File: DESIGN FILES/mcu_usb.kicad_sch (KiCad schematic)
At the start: 26 parts, among them J401 YTC-TC16S-28, Q401 MMBT3904, Q402 MMBT3904, SW401 TS-1187A-B-A-B, U401 ESP32-WROVER-E-N4R8, U402 CP2102N-A02-GQFN28R

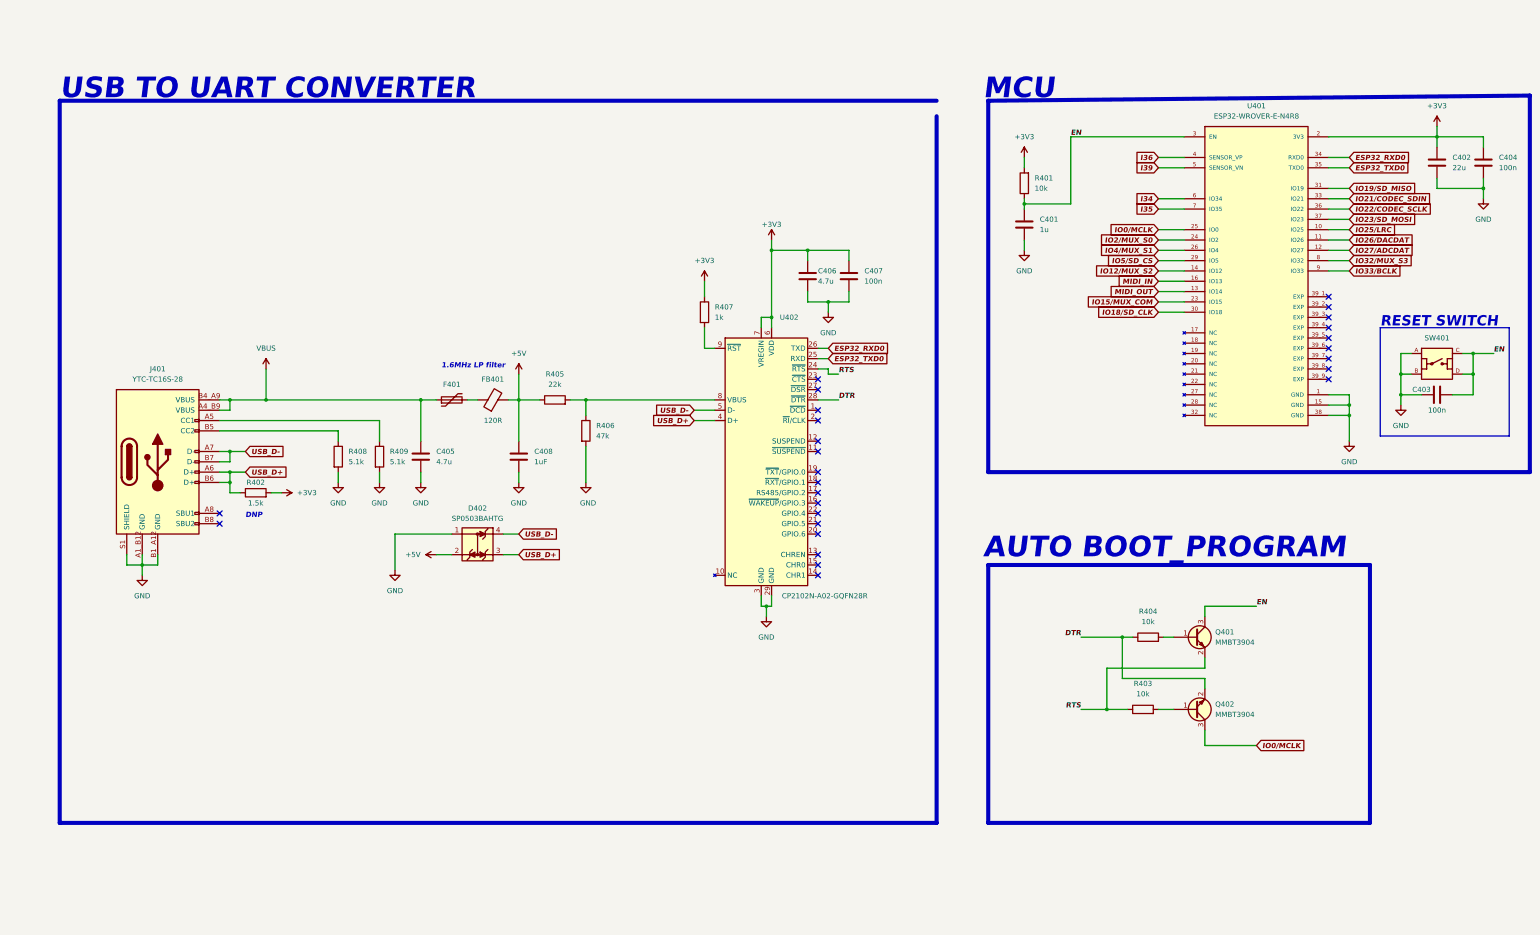
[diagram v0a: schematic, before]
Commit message: updates
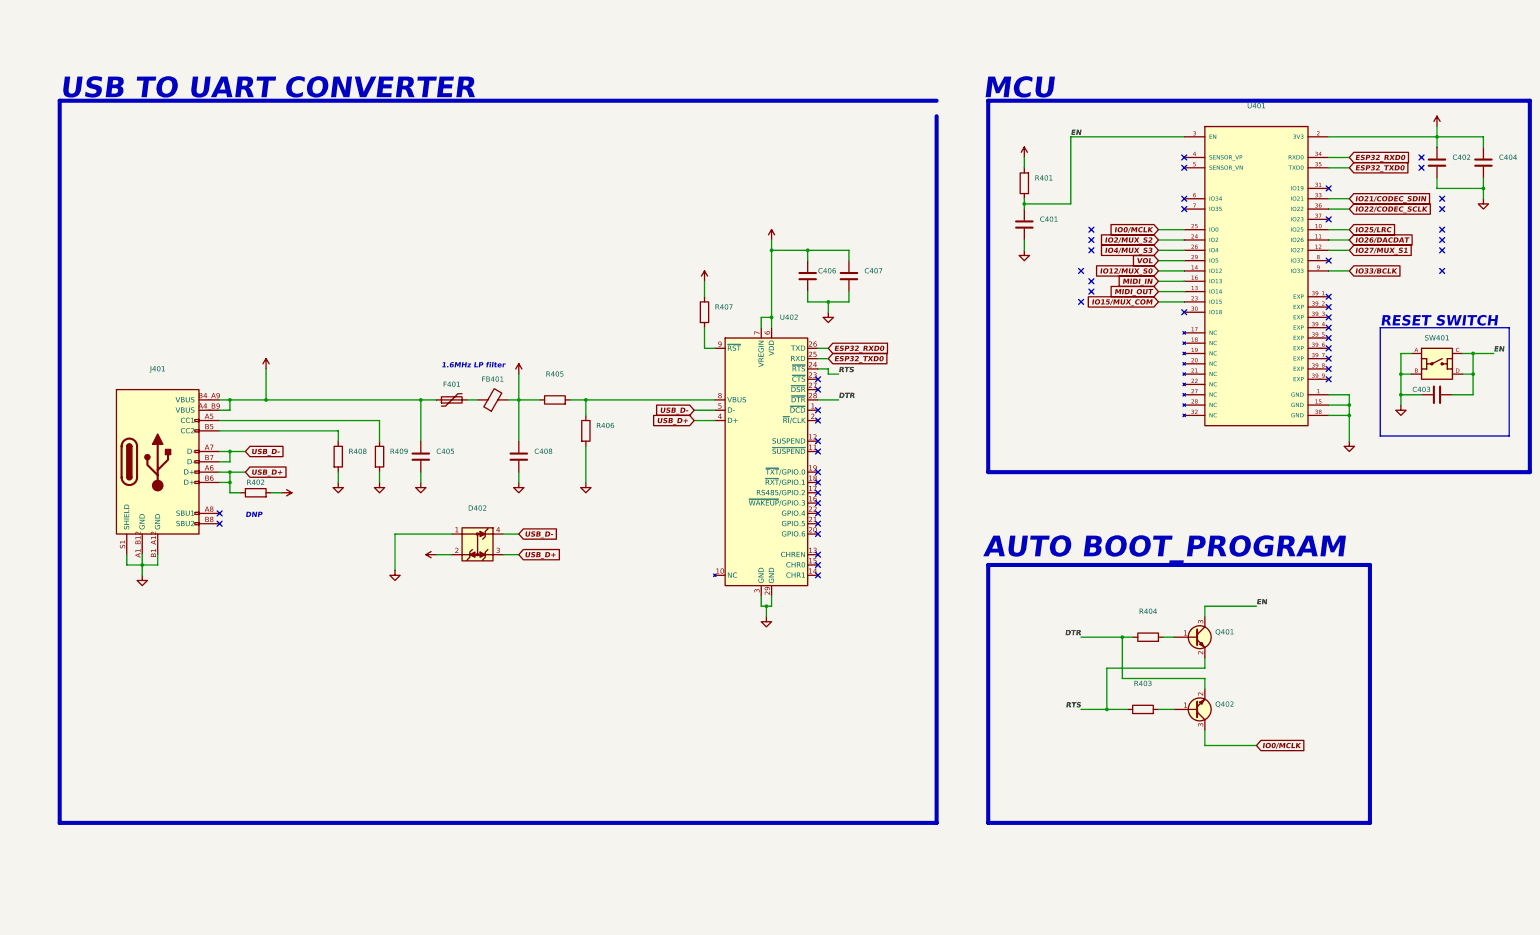
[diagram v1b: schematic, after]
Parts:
- C401: value 1u -> (none); footprint MY CAPACITOR LIBRARY:CL10A105KB8NNNC_0603 -> (none)
- C402: value 22u -> (none); footprint MY CAPACITOR LIBRARY:0603_CL10A226MQ8NRNC -> (none)
- C403, C404, C407: value 100n -> (none); footprint MY CAPACITOR LIBRARY:CC0603KRX7R9BB104_0603 -> (none)
- C405, C406: value 4.7u -> (none); footprint MY CAPACITOR LIBRARY:CL10A475KO8NNNC_0603 -> (none)
- C408: value 1uF -> (none); footprint MY CAPACITOR LIBRARY:CL10A105KB8NNNC_0603 -> (none)
- D402: value SP0503BAHTG -> (none); footprint MY DIODE LIBRARY:SP0503BAHTG_SOT-143 -> (none)
- F401: value SMD0805P020TF -> (none); footprint MY FUSE LIBRARY:0805_SMD0805P020TF -> (none)
- FB401: value 120R -> (none); footprint MY FERRITE BEAD LIBRARY:0603_BLM18AG121SN1D -> (none)
- J401: value YTC-TC16S-28 -> (none); footprint MY CONNECTOR LIBRARY:YTC-TC16S-28 -> (none)
- Q401, Q402: value MMBT3904 -> (none); footprint MY TRANSISTOR LIBRARY:MMBT3904_SOT-23 -> (none)
- R401, R403, R404: value 10k -> (none); footprint MY RESISTOR LIBRARY:0603WAF1002T5E -> (none)
- R402: value 1.5k -> (none); footprint MY RESISTOR LIBRARY:CQ03WAJ0152T5E -> (none)
- R405: value 22k -> (none); footprint MY RESISTOR LIBRARY:0603WAF2202T5E -> (none)
- R406: value 47k -> (none); footprint MY RESISTOR LIBRARY:0603WAF4702T5E -> (none)
- R407: value 1k -> (none); footprint MY RESISTOR LIBRARY:0603WAF1001T5E -> (none)
- R408, R409: value 5.1k -> (none); footprint MY RESISTOR LIBRARY:0603WAF5101T5E -> (none)
- SW401: value TS-1187A-B-A-B -> (none); footprint MY SWITCH LIBRARY:TS-1187A-B-A-B_smd -> (none)
- U401: value ESP32-WROVER-E-N4R8 -> (none); footprint MY MICROCONTROLLER LIBRARY:XCVR_ESP32-WROVER-E-N4R8 -> (none)
- U402: value CP2102N-A02-GQFN28R -> (none); footprint MY IC LIBRARY:CP2102N-A02-GQFN28R_QFN-28 -> (none)
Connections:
- net I34: no longer names the net of U401.6 (IO34)
- net I35: no longer names the net of U401.7 (IO35)
- net I36: no longer names the net of U401.4 (SENSOR_VP)
- net I39: no longer names the net of U401.5 (SENSOR_VN)
- net IO12/MUX_S2 renamed IO12/MUX_S0
- net IO18/SD_CLK: no longer names the net of U401.30 (IO18)
- net IO19/SD_MISO: no longer names the net of U401.31 (IO19)
- net IO23/SD_MOSI: no longer names the net of U401.37 (IO23)
- net IO27/ADCDAT renamed IO27/MUX_S1
- net IO2/MUX_S0 renamed IO2/MUX_S2
- net IO32/MUX_S3: no longer names the net of U401.8 (IO32)
- net IO4/MUX_S1 renamed IO4/MUX_S3
- net IO5/SD_CS renamed VOL
- no-connect marks 27 -> 50

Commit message: updates
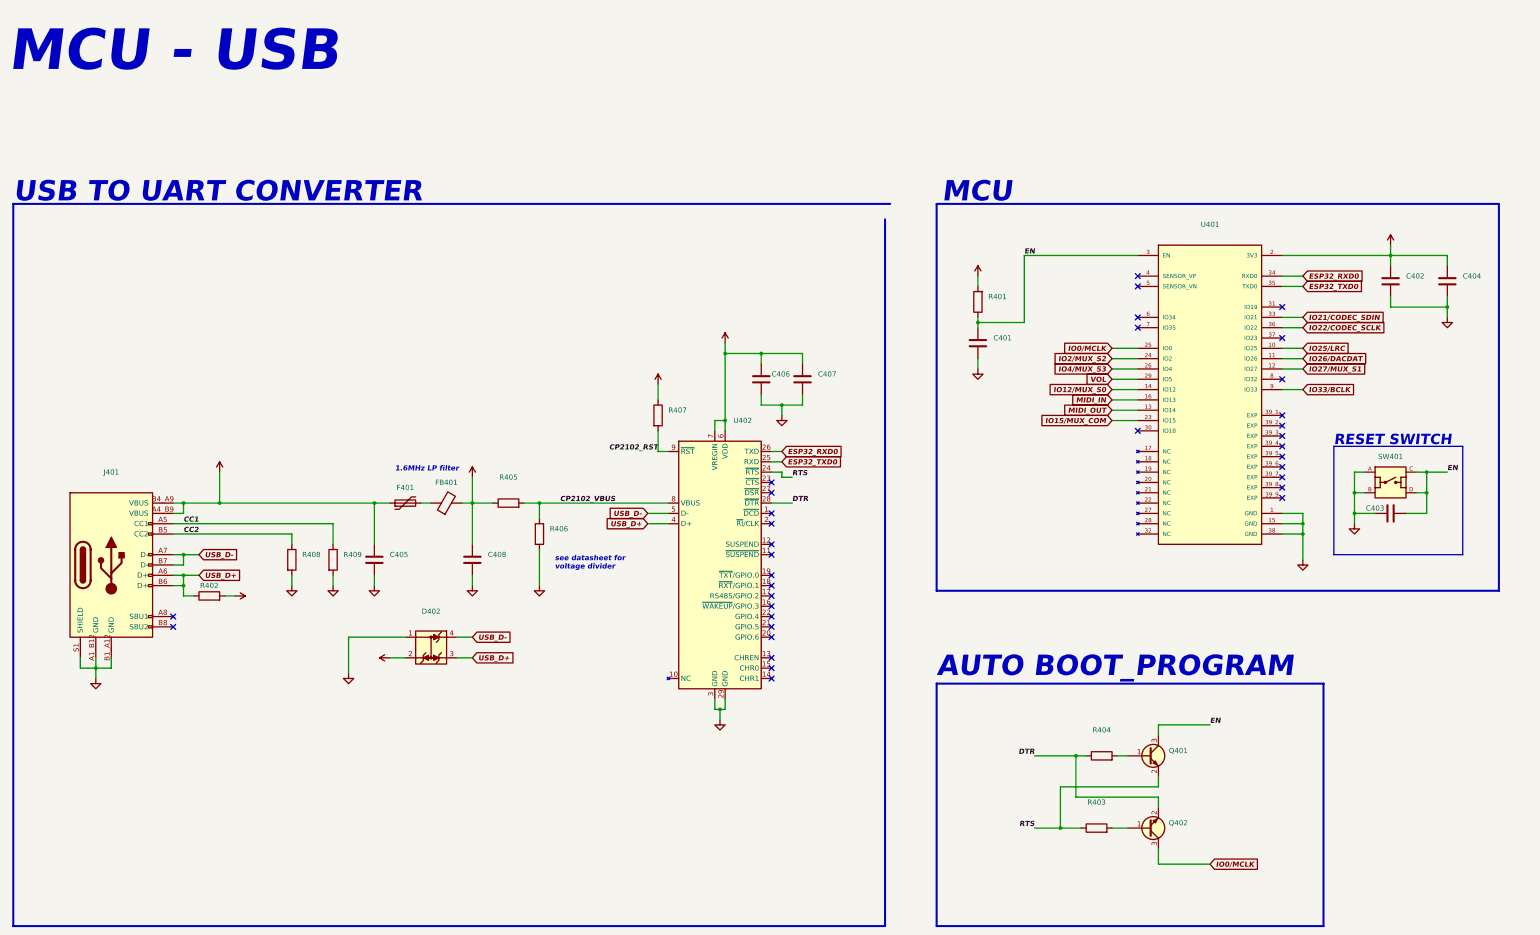
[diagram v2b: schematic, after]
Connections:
- net CC2: now reaches J401.B5 (CC2), R408.1
- net CP2102_VBUS: now reaches R405.2, R406.1, U402.8 (VBUS)
- net CP2102_RST: now reaches R407.2, U402.9 (~{RST})
- net CC1: now reaches J401.A5 (CC1), R409.1
- no-connect marks 50 -> 35
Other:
- note added: "MCU - USB"
- note added: "see datasheet for voltage divider"
- note removed: "DNP"
- company: (none) -> Joël Ucedo
- title: (none) -> ESP32 SYNTH
- moved on the sheet: C401, C402, C403, C404, C405, C406, C407, C408, D402, F401, FB401, J401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
